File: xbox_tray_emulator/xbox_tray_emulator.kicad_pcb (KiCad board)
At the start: 2 copper layers, 12.7 x 25.5 mm, 4 parts, among them J1 to Xbox, U1 ATtiny13A-S

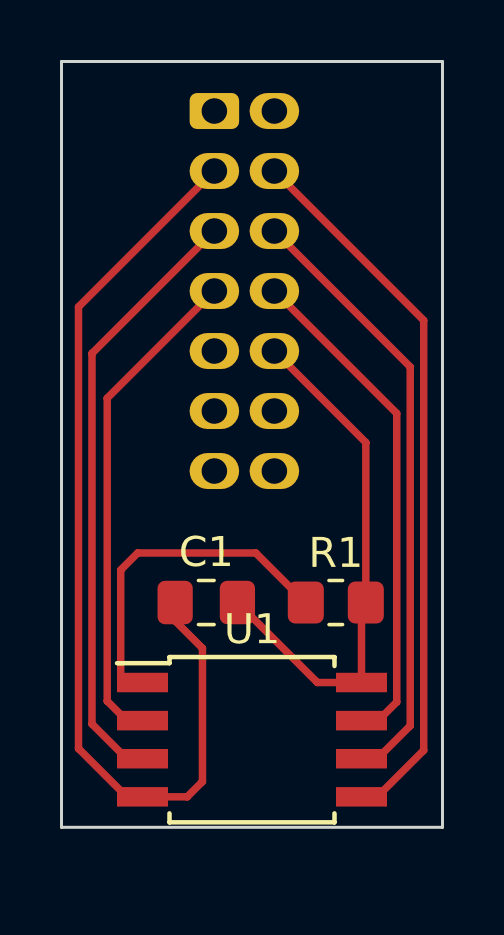
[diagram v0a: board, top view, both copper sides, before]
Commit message: add PCB
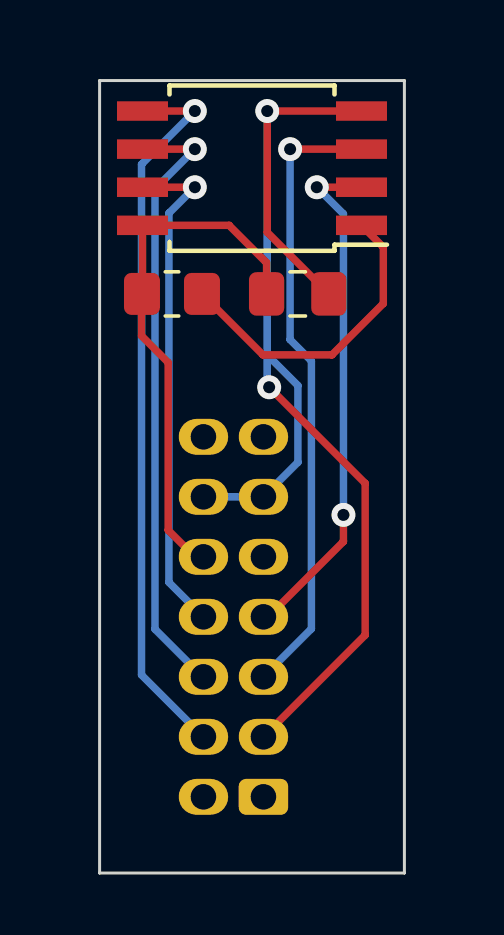
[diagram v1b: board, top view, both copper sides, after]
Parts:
- moved J1 22.9 mm to (142.6, 80.6), turned to 90 degrees
- moved U1 19.0 mm to (142.2, 59.7), turned to 180 degrees
- moved R1 11.6 mm to (139.6, 63.9), turned to 180 degrees
- moved C1 10.7 mm to (143.8, 63.9), turned to 180 degrees
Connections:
- J1 pad 11: unconnected-(J1-Pad11) -> Net-(C1-Pad1)
- J1 pad 12: unconnected-(J1-Pad12) -> Net-(C1-Pad1)
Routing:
- net Net-(C1-Pad1): track 33.0 -> 41.3 mm, vias 0 -> 2
- net Net-(R1-Pad1): track 11.6 -> 10.5 mm
- net Net-(J1-Pad5): track 20.3 -> 20.9 mm, vias 0 -> 1
- net Net-(J1-Pad6): track 20.4 -> 20.6 mm, vias 0 -> 1
- net Net-(J1-Pad4): track 24.1 -> 24.2 mm, vias 0 -> 1
- net Net-(J1-Pad8): track 16.8 -> 16.9 mm, vias 0 -> 1
- net Net-(J1-Pad7): vias 0 -> 2
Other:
- board size 12.7 x 25.5 mm -> 10.2 x 26.4 mm

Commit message: PCB cleanup
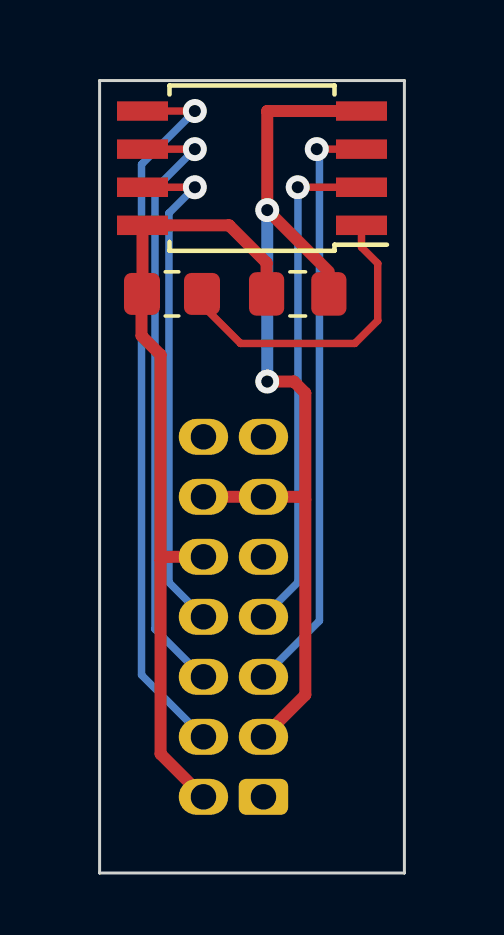
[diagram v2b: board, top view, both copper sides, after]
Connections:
- J1 pad 2: unconnected-(J1-Pad2) -> Net-(C1-Pad2)
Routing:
- net Net-(C1-Pad2): track 17.7 -> 27.1 mm
- net Net-(C1-Pad1): track 41.3 -> 32.7 mm
- net Net-(J1-Pad5): track 20.9 -> 19.9 mm
- net Net-(J1-Pad7): track 17.4 -> 16.9 mm, vias 2 -> 1
